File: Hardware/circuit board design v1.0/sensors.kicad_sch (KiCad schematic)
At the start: 6 parts, among them U4 BME280

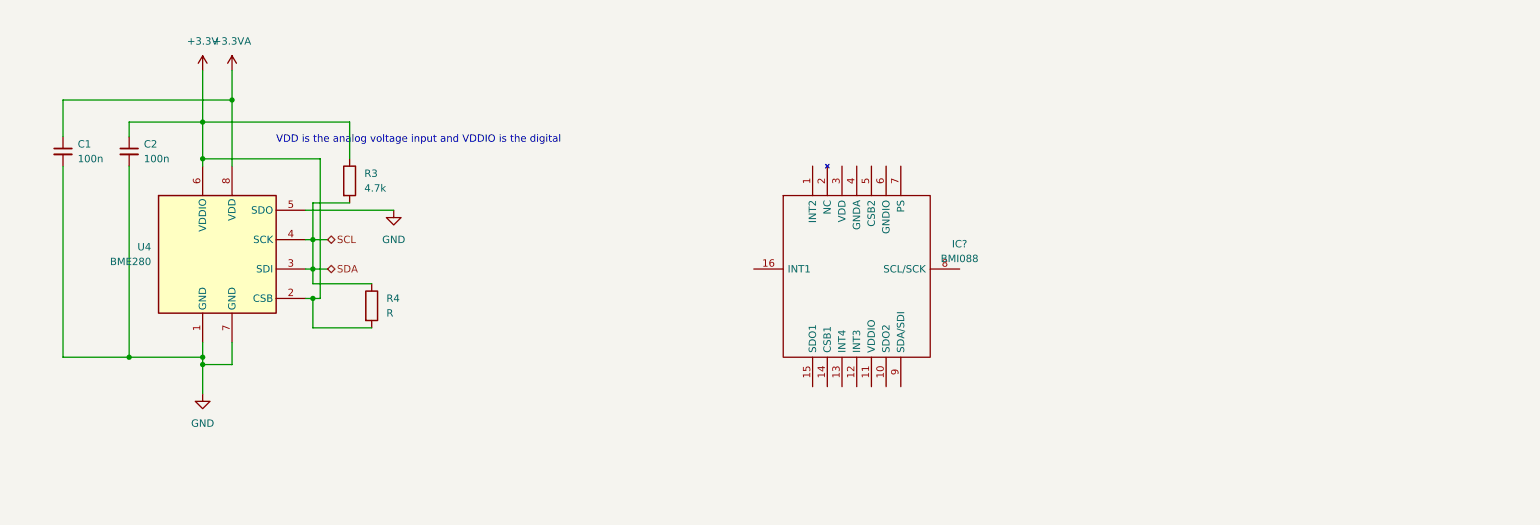
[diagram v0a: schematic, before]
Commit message: Continued layout for PCB
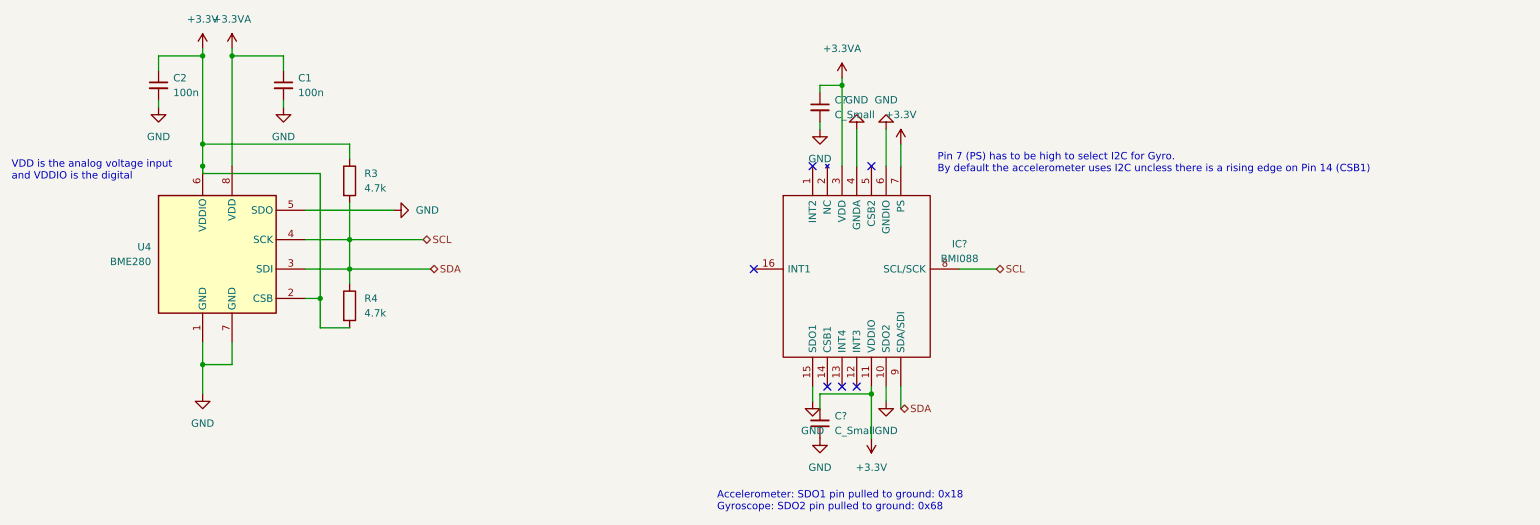
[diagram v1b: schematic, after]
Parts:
- added C? (x2): C_Small, Capacitor_SMD:C_0603_1608Metric, symbol Device:C_Small
- C1: footprint (none) -> Capacitor_SMD:C_0603_1608Metric
- C2: footprint Capacitor_SMD:C_0603_1608Metric_Pad1.08x0.95mm_HandSolder -> Capacitor_SMD:C_0603_1608Metric
- R3: footprint (none) -> Resistor_SMD:R_0603_1608Metric
- R4: value R -> 4.7k; footprint (none) -> Resistor_SMD:R_0603_1608Metric
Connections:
- net +3.3V: now also IC?.11 (VDDIO), IC?.7 (PS), C?.2
- net +3.3VA: now also IC?.3 (VDD), C?.1
- net GND: now also IC?.10 (SDO2), IC?.15 (SDO1), IC?.4 (GNDA), IC?.6 (GNDIO), C?.1, C?.2
- net SCL: now also IC?.8 (SCL/SCK), IC?.9 (SDA/SDI)
- no-connect marks 0 -> 6
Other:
- note added: "Accelerometer: SDO1 pin pulled to ground: 0x18 Gyroscope: SDO2 pin pulled to ground: 0x68"
- note added: "Pin 7 (PS) has to be high to select I2C for Gyro. By default the accelerometer uses I2C uncless there is a rising edge on Pin 14 (CSB1)"
- moved on the sheet: C1, C2, R4
